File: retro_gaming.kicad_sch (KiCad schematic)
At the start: 58 parts, among them J6 Output Speaker, SW1 UP, SW10 L2, SW11 R1, SW12 R2, SW13 Start, SW14 Select, SW2 Left, SW3 Right, SW4 Down, SW5 Y, SW6 X, SW7 B, SW8 A, SW9 L1, U1 ADS1015IDGS, U2 TPS61230ARNST, U3 MAX98357AETE_T, U4 TPS60501DGS, U5 BQ25895RTWR, U6 TS3USB221RSER

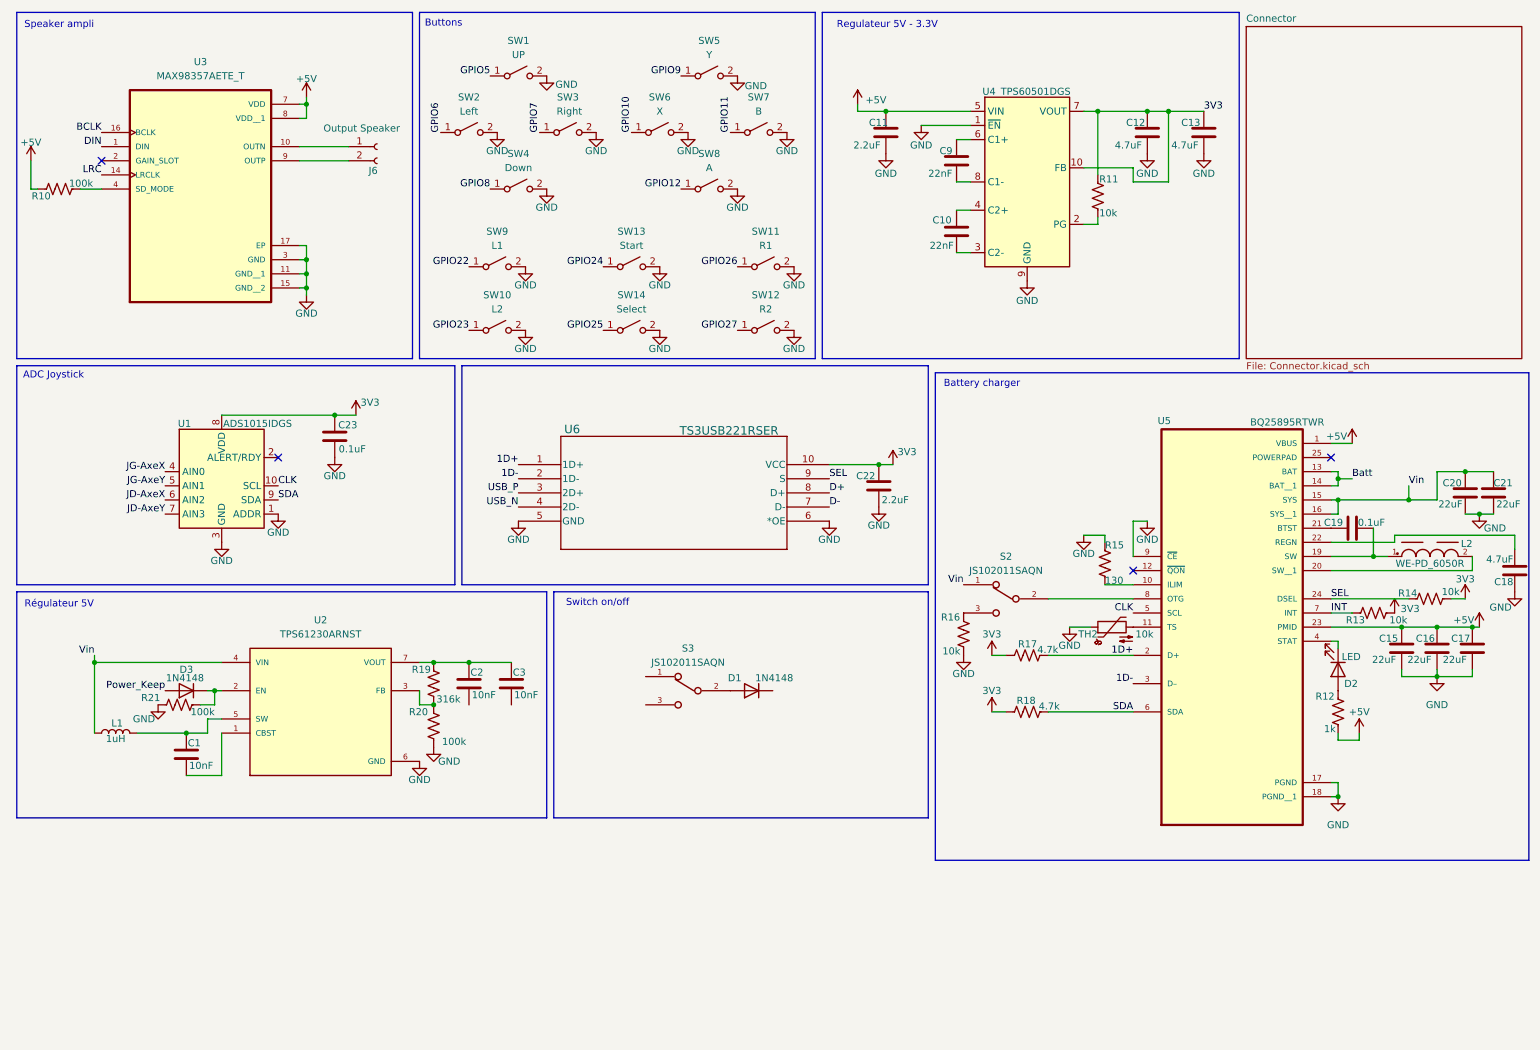
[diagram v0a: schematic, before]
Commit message: Review B
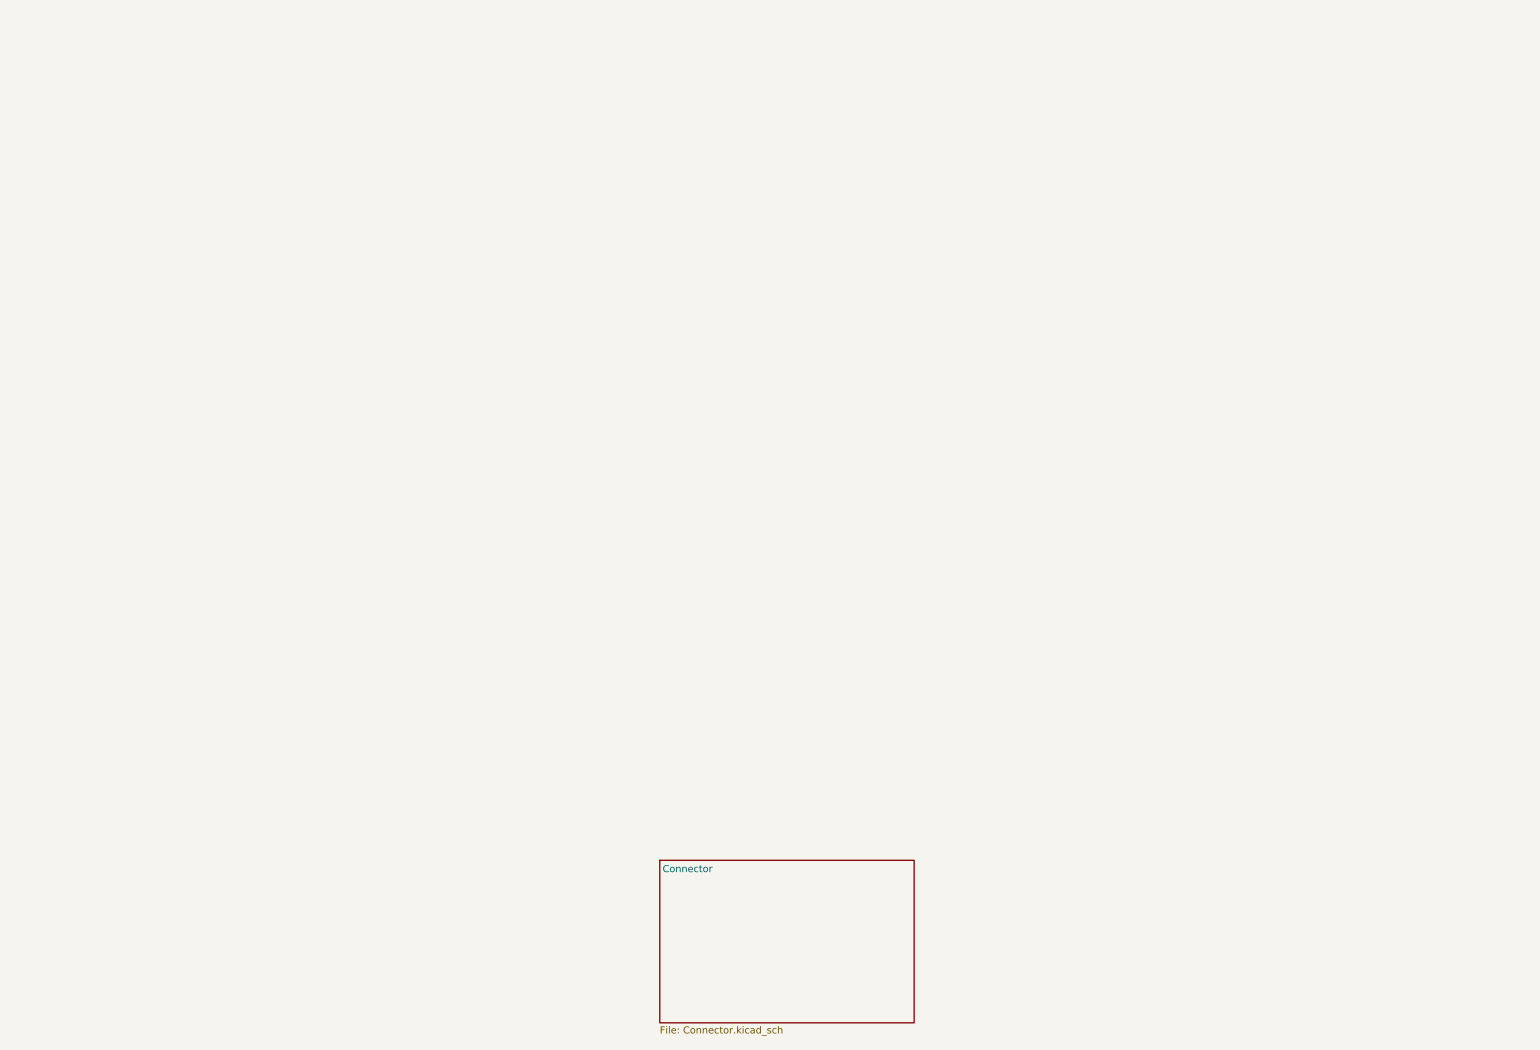
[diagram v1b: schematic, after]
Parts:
- removed C1, C2, C3: 10nF, symbol Device:C
- removed C10, C9: 22nF, symbol Device:C
- removed C11, C22: 2.2uF, symbol Device:C
- removed C12, C13, C18: 4.7uF, symbol Device:C
- removed C15, C16, C17, C20, C21: 22uF, symbol Device:C
- removed C19, C23: 0.1uF, symbol Device:C
- removed D1, D3: 1N4148, Diode_THT:D_DO-35_SOD27_P7.62mm_Horizontal, symbol Diode:1N4148
- removed D2: LED, symbol Device:LED
- removed J6: Output Speaker, Connector_PinSocket_2.54mm:PinSocket_1x02_P2.54mm_Vertical, symbol Connector:Conn_01x02_Socket
- removed L1: 1uH, symbol Device:L
- removed L2: WE-PD_6050R, 7447786002:WE-PD_6050R, symbol WE-PD_6050R:WE-PD_6050R
- removed R10, R20, R21: 100k, symbol Device:R_US
- removed R11, R13, R14, R16: 10k, symbol Device:R_US
- removed R12: 1k, symbol Device:R_US
- removed R15: 130, symbol Device:R_US
- removed R17, R18: 4.7k, symbol Device:R_US
- removed R19: 316k, symbol Device:R_US
- removed S2, S3: JS102011SAQN, JS102011SAQN:SW_JS102011SAQN, symbol JS102011SAQN:JS102011SAQN
- removed SW1: UP, symbol Switch:SW_SPST
- removed SW10: L2, symbol Switch:SW_SPST
- removed SW11: R1, symbol Switch:SW_SPST
- removed SW12: R2, symbol Switch:SW_SPST
- removed SW13: Start, symbol Switch:SW_SPST
- removed SW14: Select, symbol Switch:SW_SPST
- removed SW2: Left, symbol Switch:SW_SPST
- removed SW3: Right, symbol Switch:SW_SPST
- removed SW4: Down, symbol Switch:SW_SPST
- removed SW5: Y, symbol Switch:SW_SPST
- removed SW6: X, symbol Switch:SW_SPST
- removed SW7: B, symbol Switch:SW_SPST
- removed SW8: A, symbol Switch:SW_SPST
- removed SW9: L1, symbol Switch:SW_SPST
- removed TH2: 10k, symbol Device:Thermistor_NTC
- removed U1: ADS1015IDGS, Package_SO:TSSOP-10_3x3mm_P0.5mm, symbol Analog_ADC:ADS1015IDGS
- removed U2: TPS61230ARNST, TPS61230ARNST:IC_TPS61230ARNST, symbol TPS61230ARNST:TPS61230ARNST
- removed U3: MAX98357AETE_T, MAX98357AETE_T:QFN50P300X300X80-17N, symbol MAX98357AETE_T:MAX98357AETE_T
- removed U4: TPS60501DGS, Package_SO:MSOP-10_3x3mm_P0.5mm, symbol Regulator_SwitchedCapacitor:TPS60501DGS
- removed U5: BQ25895RTWR, BQ25895RTWR:QFN50P400X400X80-25N, symbol BQ25895RTWR:BQ25895RTWR
- removed U6: TS3USB221RSER, TS3USB221RSER:RSE10, symbol TS3USB221RSER:TS3USB221RSER
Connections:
- no-connect marks 4 -> 0
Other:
- note removed: "ADC Joystick"
- note removed: "Battery charger"
- note removed: "Buttons"
- note removed: "Regulateur 5V - 3.3V"
- note removed: "Régulateur 5V"
- note removed: "Speaker ampli"
- note removed: "Switch on/off"
- title: (none) -> Retro console 

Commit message: Review B
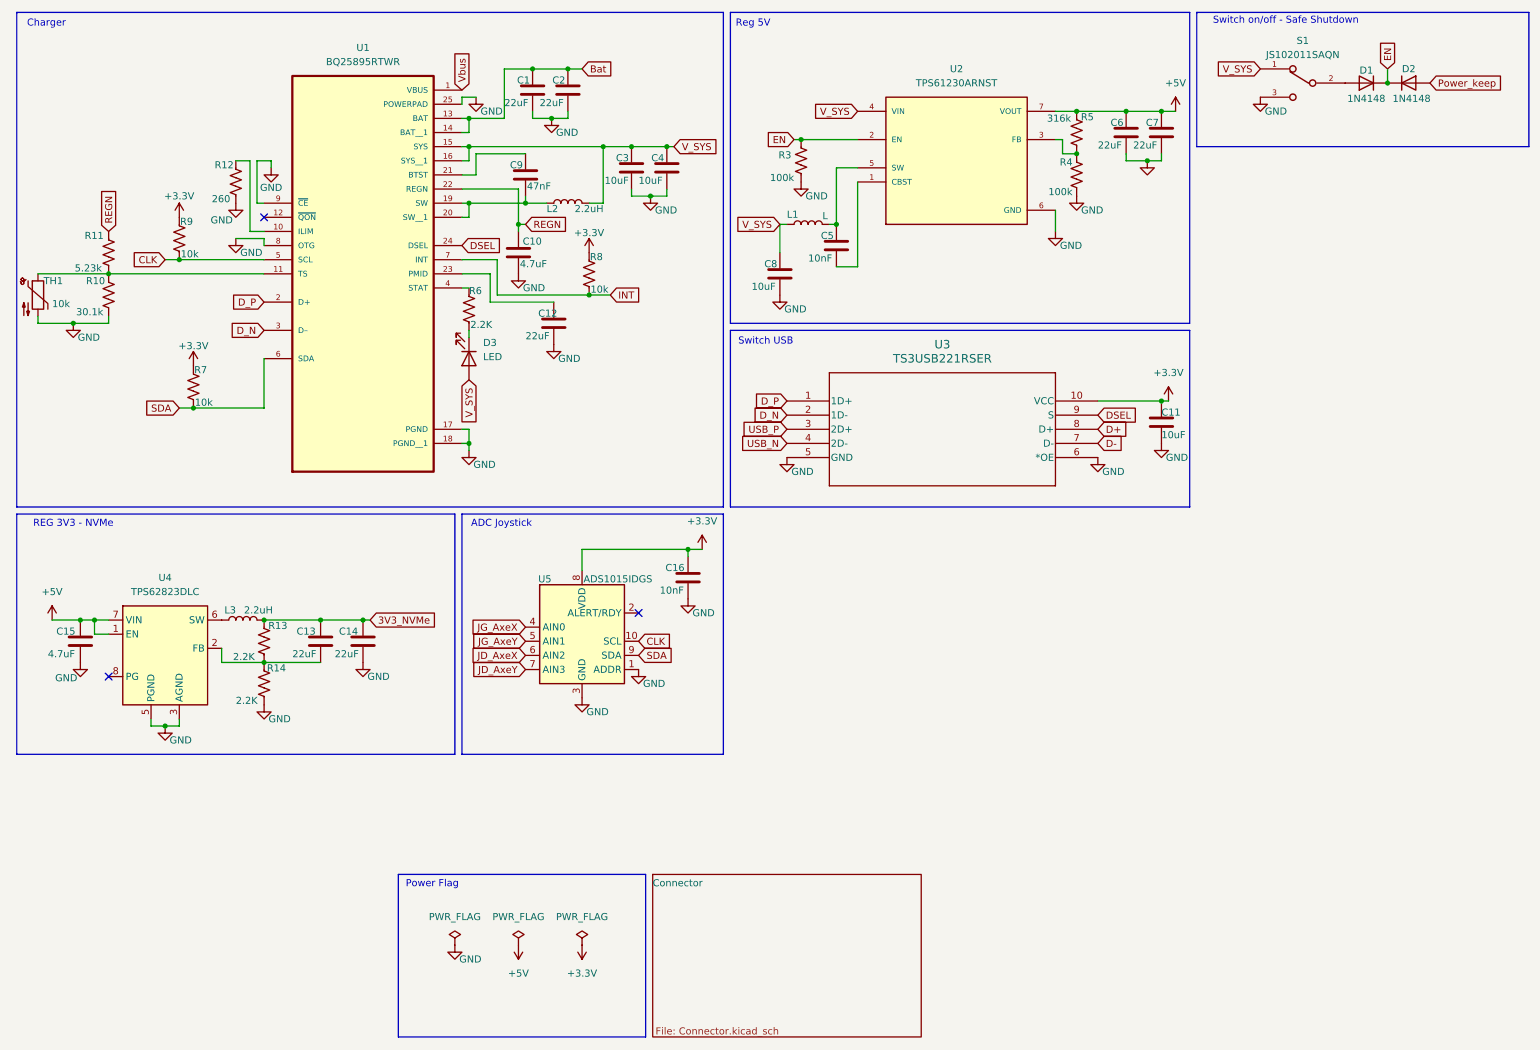
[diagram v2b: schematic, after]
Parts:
- added C1, C12, C13, C14, C2, C6, C7: 22uF, symbol Device:C
- added C10, C15: 4.7uF, symbol Device:C
- added C11, C3, C4, C8: 10uF, symbol Device:C
- added C16, C5: 10nF, symbol Device:C
- added C9: 47nF, symbol Device:C
- added D1, D2: 1N4148, Diode_THT:D_DO-35_SOD27_P7.62mm_Horizontal, symbol Diode:1N4148
- added D3: LED, symbol Device:LED
- added L1: L, symbol Device:L
- added L2, L3: 2.2uH, symbol Device:L
- added R10: 30.1k, symbol Device:R_US
- added R11: 5.23k, symbol Device:R_US
- added R12: 260, symbol Device:R_US
- added R13, R14, R6: 2.2K, symbol Device:R_US
- added R3, R4: 100k, symbol Device:R_US
- added R5: 316k, symbol Device:R_US
- added R7, R8, R9: 10k, symbol Device:R_US
- added S1: JS102011SAQN, JS102011SAQN:SW_JS102011SAQN, symbol Switch:JS102011SAQN
- added TH1: 10k, symbol Device:Thermistor_NTC
- added U1: BQ25895RTWR, BQ25895RTWR:QFN50P400X400X80-25N, symbol BQ25895RTWR:BQ25895RTWR
- added U2: TPS61230ARNST, TPS61230ARNST:IC_TPS61230ARNST, symbol TPS61230ARNST:TPS61230ARNST
- added U3: TS3USB221RSER, RSE10, symbol TS3USB221RSER:TS3USB221RSER
- added U4: TPS62823DLC, Package_SON:Texas_VSON-HR-8_1.5x2mm_P0.5mm, symbol Regulator_Switching:TPS62823DLC
- added U5: ADS1015IDGS, Package_SO:TSSOP-10_3x3mm_P0.5mm, symbol Analog_ADC:ADS1015IDGS
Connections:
- new net: R10.1, R11.2, TH1.1, U1.11 (TS)
- new net: R6.1, U1.4 (STAT)
- new net: D3.1 (K), R6.2
- new net: D1.2 (A), S1.2
- new net: C12.1, U1.23 (PMID)
- new net: R12.1, U1.10 (ILIM)
- new net: C9.2, L2.1, U1.19 (SW), U1.20 (SW__1)
- new net: C9.1, U1.21 (BTST)
- new net: C13.2, R13.2, R14.1, U4.2 (FB)
- new net: C5.2, U2.1 (CBST)
- new net: R4.1, R5.2, U2.3 (FB)
- new net: C5.1, L1.2, U2.5 (SW)
- new net: L3.1, U4.6 (SW)
- new net +3.3V: C11.1, C16.1, R7.1, R8.1, R9.1, U3.10 (VCC), U5.8 (VDD)
- new net +5V: C15.1, C6.1, C7.1, R5.1, U2.7 (VOUT), U4.1 (EN), U4.7 (VIN)
- new net 3V3_NVMe: C13.1, C14.1, L3.2, R13.1
- new net Bat: C1.1, C2.1, U1.13 (BAT), U1.14 (BAT__1)
- new net CLK: R9.2, U1.5 (SCL), U5.10 (SCL)
- new net D+: U3.8 (D+)
- new net D-: U3.7 (D-)
- new net DSEL: U1.24 (DSEL), U3.9 (S)
- new net D_N: U1.3 (D–), U3.2 (1D-)
- new net D_P: U1.2 (D+), U3.1 (1D+)
- new net EN: D1.1 (K), D2.1 (K), R3.1, U2.2 (EN)
- new net GND: C1.2, C10.2, C11.2, C12.2, C14.2, C15.2, C16.2, C2.2, C3.2, C4.2, C6.2, C7.2, C8.2, R10.2, R12.2, R14.2, R3.2, R4.2, S1.3, TH1.2, U1.17 (PGND), U1.18 (PGND__1), U1.25 (POWERPAD), U1.8 (OTG), U1.9 (~{CE}), U2.6 (GND), U3.5 (GND), U3.6 (*OE), U4.3 (AGND), U4.5 (PGND), U5.1 (ADDR), U5.3 (GND)
- new net INT: R8.2, U1.7 (INT)
- new net JD_AxeX: U5.6 (AIN2)
- new net JD_AxeY: U5.7 (AIN3)
- new net JG_AxeX: U5.4 (AIN0)
- new net JG_AxeY: U5.5 (AIN1)
- new net Power_keep: D2.2 (A)
- new net REGN: C10.1, R11.1, U1.22 (REGN)
- new net SDA: R7.2, U1.6 (SDA), U5.9 (SDA)
- new net USB_N: U3.4 (2D-)
- new net USB_P: U3.3 (2D+)
- new net V_SYS: C3.1, C4.1, C8.1, D3.2 (A), L1.1, L2.2, S1.1, U1.15 (SYS), U1.16 (SYS__1), U2.4 (VIN)
- new net Vbus: U1.1 (VBUS)
- no-connect marks 0 -> 3
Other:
- note added: "ADC Joystick"
- note added: "Charger"
- note added: "Power Flag"
- note added: "REG 3V3 - NVMe"
- note added: "Reg 5V"
- note added: "Switch USB"
- note added: "Switch on/off - Safe Shutdown"

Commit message: Final Schematic
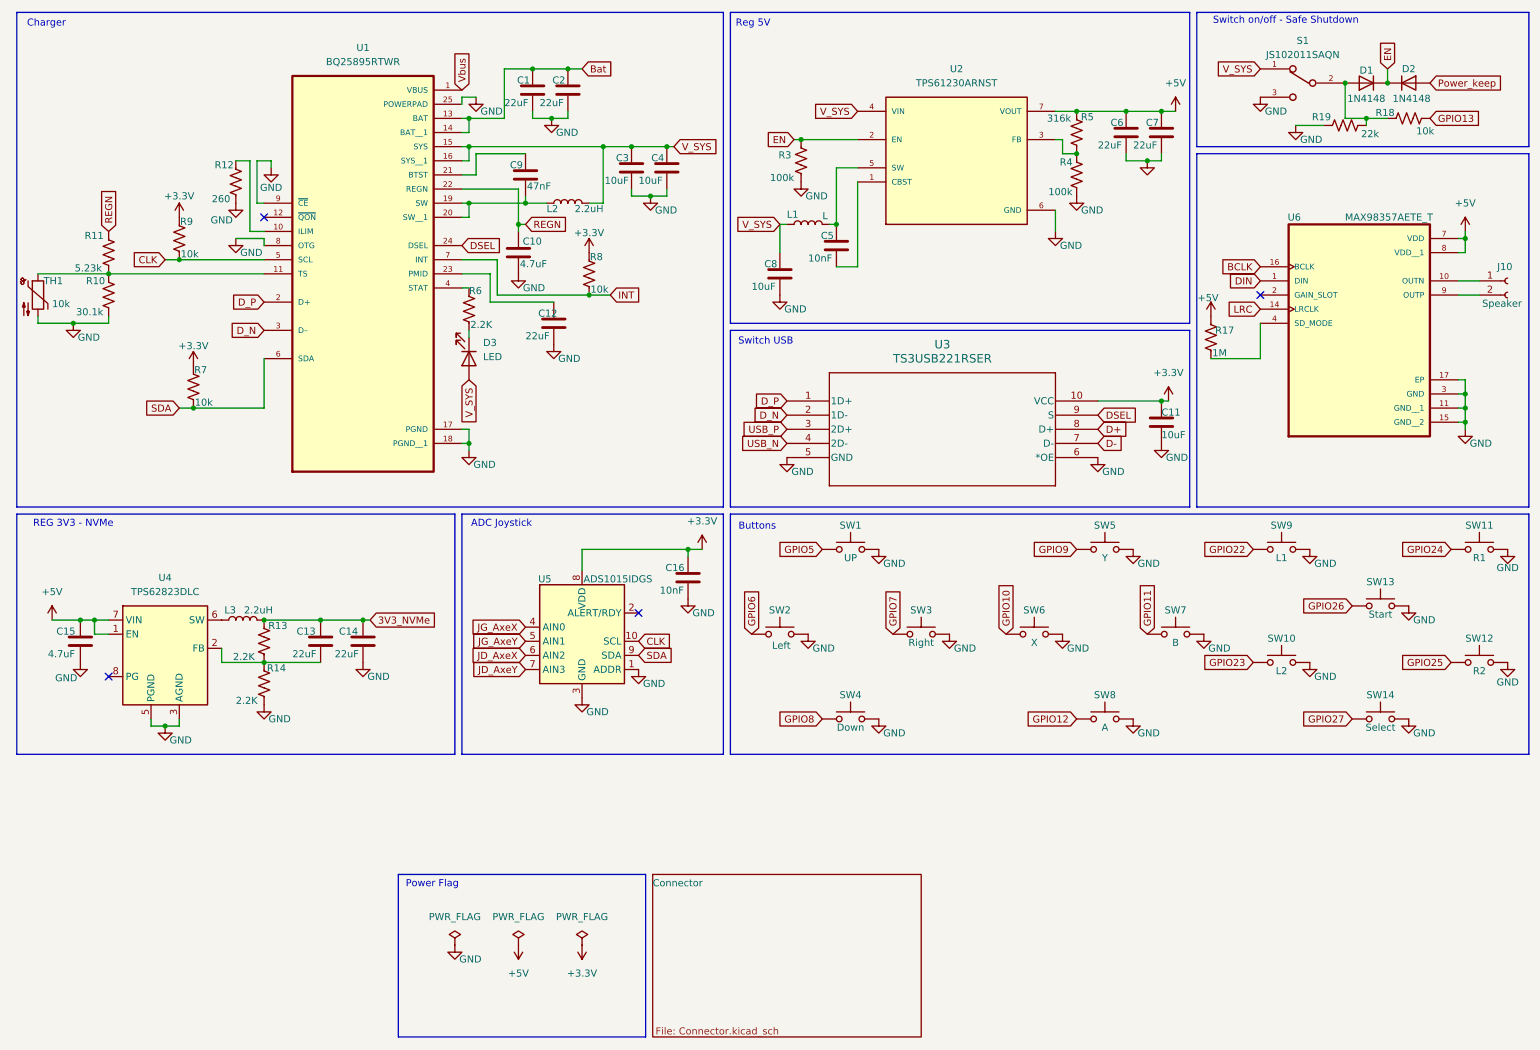
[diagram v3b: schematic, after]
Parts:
- added J10: Speaker, symbol Connector:Conn_01x02_Socket
- added R17: 1M, symbol Device:R_US
- added R18: 10k, symbol Device:R_US
- added R19: 22k, symbol Device:R_US
- added SW1: UP, symbol Switch:SW_Push
- added SW10: L2, symbol Switch:SW_Push
- added SW11: R1, symbol Switch:SW_Push
- added SW12: R2, symbol Switch:SW_Push
- added SW13: Start, symbol Switch:SW_Push
- added SW14: Select, symbol Switch:SW_Push
- added SW2: Left, symbol Switch:SW_Push
- added SW3: Right, symbol Switch:SW_Push
- added SW4: Down, symbol Switch:SW_Push
- added SW5: Y, symbol Switch:SW_Push
- added SW6: X, symbol Switch:SW_Push
- added SW7: B, symbol Switch:SW_Push
- added SW8: A, symbol Switch:SW_Push
- added SW9: L1, symbol Switch:SW_Push
- added U6: MAX98357AETE_T, MAX98357AETE_T:QFN50P300X300X80-17N, symbol MAX98357AETE_T:MAX98357AETE_T
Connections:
- net +5V: now also R17.1, U6.7 (VDD), U6.8 (VDD__1)
- net GND: now also R19.1, SW1.2, SW10.2, SW11.2, SW12.2, SW13.2, SW14.2, SW2.2, SW3.2, SW4.2, SW5.2, SW6.2, SW7.2, SW8.2, SW9.2, U6.11 (GND__1), U6.15 (GND__2), U6.17 (EP), U6.3 (GND)
- net at D1.2 (A), S1.2: now also R18.1, R19.2
- new net: R17.2, U6.4 (SD_MODE)
- new net: J10.1 (Pin_1), U6.10 (OUTN)
- new net: J10.2 (Pin_2), U6.9 (OUTP)
- new net BCLK: U6.16 (BCLK)
- new net DIN: U6.1 (DIN)
- new net GPIO10: SW6.1
- new net GPIO11: SW7.1
- new net GPIO12: SW8.1
- new net GPIO13: R18.2
- new net GPIO22: SW9.1
- new net GPIO23: SW10.1
- new net GPIO24: SW11.1
- new net GPIO25: SW12.1
- new net GPIO26: SW13.1
- new net GPIO27: SW14.1
- new net GPIO5: SW1.1
- new net GPIO6: SW2.1
- new net GPIO7: SW3.1
- new net GPIO8: SW4.1
- new net GPIO9: SW5.1
- new net LRC: U6.14 (LRCLK)
- no-connect marks 3 -> 4
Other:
- note added: "Buttons"
